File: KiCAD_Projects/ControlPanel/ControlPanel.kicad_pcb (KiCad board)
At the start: 2 copper layers, 0 parts

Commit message: 4.0発注かけた｡テレメトリとコンパネ作る
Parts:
- added D1: LED, LEDs:LED-3MM, F.Cu at (29.2, 3.81)
- added D2: LED, LEDs:LED-3MM, F.Cu at (24.1, 6.35)
- added D3: LED, LEDs:LED-3MM, F.Cu at (29.2, 8.89)
- added D4: LED, LEDs:LED-3MM, F.Cu at (24.1, 11.4)
- added D5: LED, LEDs:LED-3MM, F.Cu at (29.2, 14.0)
- added D6: LED, LEDs:LED-3MM, F.Cu at (24.1, 16.5)
- added D7: LED, LEDs:LED-3MM, F.Cu at (29.2, 19.1)
- added D8: LED, LEDs:LED-3MM, F.Cu at (24.1, 21.6)
- added R1: R, RP_KiCAD_Libs:C1608_WP, B.Cu at (19.1, 3.81)
- added R2: R, RP_KiCAD_Libs:C1608_WP, B.Cu at (19.1, 6.35)
- added R3: R, RP_KiCAD_Libs:C1608_WP, B.Cu at (19.1, 8.89)
- added R4: R, RP_KiCAD_Libs:C1608_WP, B.Cu at (19.1, 11.4)
- added R5: R, RP_KiCAD_Libs:C1608_WP, B.Cu at (19.1, 14.0)
- added R6: R, RP_KiCAD_Libs:C1608_WP, B.Cu at (19.1, 16.5)
- added R7: R, RP_KiCAD_Libs:C1608_WP, B.Cu at (19.1, 19.1)
- added R8: R, RP_KiCAD_Libs:C1608_WP, B.Cu at (19.1, 21.6)
- added SW1: SWITCH_INV, Buttons_Switches_ThroughHole:SW_toggle_3P, F.Cu at (78.7, 2.54)
- added SW2: SWITCH_INV, Buttons_Switches_ThroughHole:SW_toggle_3P, F.Cu at (78.7, 7.62)
- added SW3: SWITCH_INV, Buttons_Switches_ThroughHole:SW_toggle_3P, F.Cu at (78.7, 12.7)
- added SW4: SWITCH_INV, Buttons_Switches_ThroughHole:SW_toggle_3P, F.Cu at (78.7, 17.8)
- added SW5: SWITCH_INV, Buttons_Switches_ThroughHole:SW_toggle_3P, F.Cu at (78.7, 22.9)
- added SW6: SWITCH_INV, Buttons_Switches_ThroughHole:SW_toggle_3P, F.Cu at (78.7, 27.9)
- added SW7: SWITCH_INV, Buttons_Switches_ThroughHole:SW_toggle_3P, F.Cu at (78.7, 33.0)
- added SW8: SWITCH_INV, Buttons_Switches_ThroughHole:SW_toggle_3P, F.Cu at (78.7, 38.1)
- added U1: F103_mini, RP_KiCAD_Libs:F103_mini, F.Cu at (48.3, 25.4)
- added U2: SW_ROTARY_16, Buttons_Switches_ThroughHole:rotary_0F, F.Cu at (22.9, 31.8)
- added U3: SW_ROTARY_16, Buttons_Switches_ThroughHole:rotary_0F, F.Cu at (22.9, 43.2)
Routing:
- net GND: track 0.00 -> 166.6 mm
- net /TOGGLE_H: track 0.00 -> 28.1 mm
- net /TOGGLE_G: track 0.00 -> 25.6 mm
- net /TOGGLE_F: track 0.00 -> 22.3 mm
- net /TOGGLE_E: track 0.00 -> 21.2 mm
- net /TOGGLE_D: track 0.00 -> 20.2 mm
- net /TOGGLE_C: track 0.00 -> 19.1 mm
- net /TOGGLE_B: track 0.00 -> 18.1 mm
- net /TOGGLE_A: track 0.00 -> 18.1 mm
- net /ROTARY_B4: track 0.00 -> 17.1 mm
- net /ROTARY_A4: track 0.00 -> 16.6 mm
- net /ROTARY_B1: track 0.00 -> 16.1 mm
- net /ROTARY_A1: track 0.00 -> 15.5 mm
- net /ROTARY_B8: track 0.00 -> 11.0 mm
- net /ROTARY_A8: track 0.00 -> 10.5 mm
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- added copper zone on B.Cu, net (none)
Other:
- board outline added: 100 x 50 mm

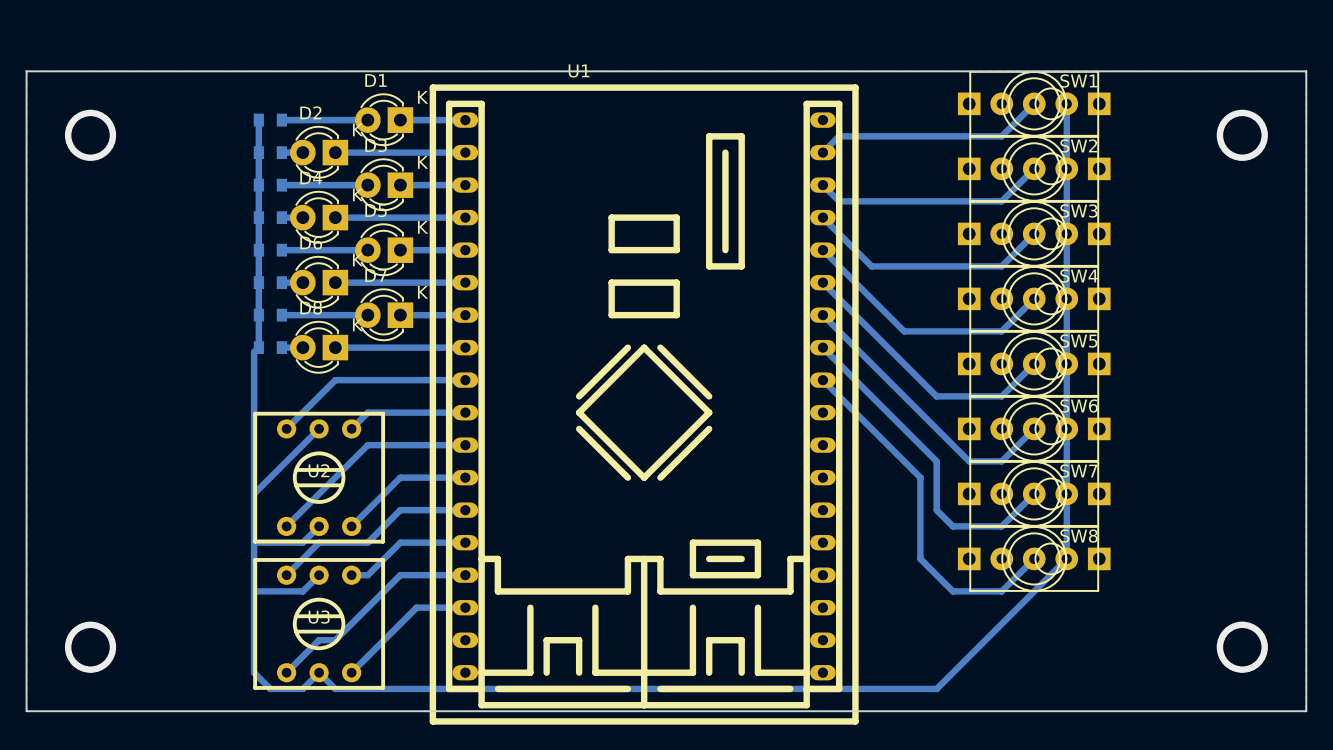
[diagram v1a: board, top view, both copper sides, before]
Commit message: コンパネおわり｡キャンサー作る
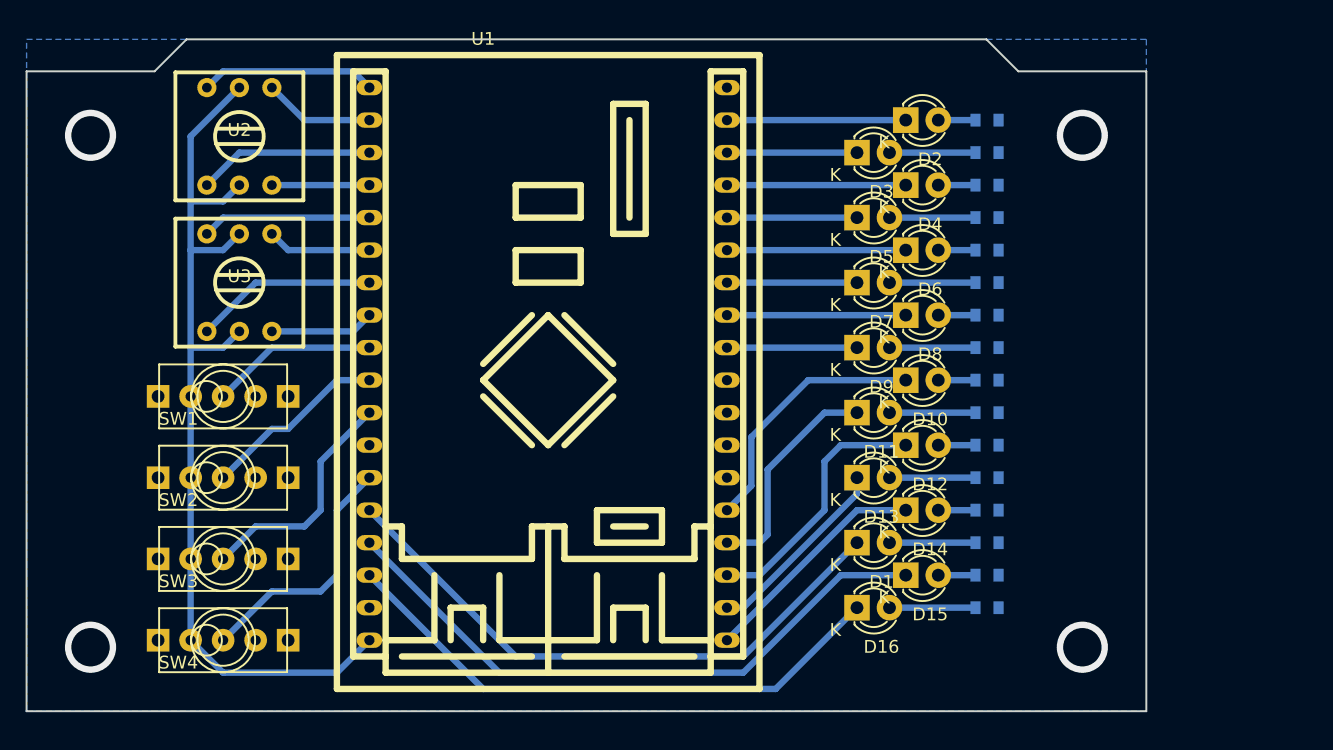
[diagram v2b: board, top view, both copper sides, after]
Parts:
- removed SW5, SW6, SW7, SW8: SWITCH_INV, Buttons_Switches_ThroughHole:SW_toggle_3P
- added D10: LED, LEDs:LED-3MM, F.Cu at (68.7, 24.1)
- added D11: LED, LEDs:LED-3MM, F.Cu at (64.9, 26.7)
- added D12: LED, LEDs:LED-3MM, F.Cu at (68.7, 29.2)
- added D13: LED, LEDs:LED-3MM, F.Cu at (64.9, 31.8)
- added D14: LED, LEDs:LED-3MM, F.Cu at (68.7, 34.3)
- added D15: LED, LEDs:LED-3MM, F.Cu at (68.7, 39.4)
- added D16: LED, LEDs:LED-3MM, F.Cu at (64.9, 41.9)
- added D9: LED, LEDs:LED-3MM, F.Cu at (64.9, 21.6)
- added R10: R, RP_KiCAD_Libs:C1608_WP, B.Cu at (75.0, 24.1)
- added R11: R, RP_KiCAD_Libs:C1608_WP, B.Cu at (75.0, 26.7)
- added R12: R, RP_KiCAD_Libs:C1608_WP, B.Cu at (75.0, 29.2)
- added R13: R, RP_KiCAD_Libs:C1608_WP, B.Cu at (75.0, 31.8)
- added R14: R, RP_KiCAD_Libs:C1608_WP, B.Cu at (75.0, 34.3)
- added R15: R, RP_KiCAD_Libs:C1608_WP, B.Cu at (75.0, 39.4)
- added R16: R, RP_KiCAD_Libs:C1608_WP, B.Cu at (75.0, 41.9)
- added R9: R, RP_KiCAD_Libs:C1608_WP, B.Cu at (75.0, 21.6)
- moved SW4 68.8 mm to (15.4, 44.5), turned to 180 degrees
- moved SW3 68.3 mm to (15.4, 38.1), turned to 180 degrees
- moved SW2 67.8 mm to (15.4, 31.8), turned to 180 degrees
- moved SW1 67.4 mm to (15.4, 25.4), turned to 180 degrees
- moved R1 65.0 mm to (75.0, 36.8), turned to 180 degrees
- moved R2 56.1 mm to (75.0, 3.81), turned to 180 degrees
- moved R3 56.1 mm to (75.0, 6.35), turned to 180 degrees
- moved R4 56.1 mm to (75.0, 8.89), turned to 180 degrees
- moved R5 56.1 mm to (75.0, 11.4), turned to 180 degrees
- moved R6 56.1 mm to (75.0, 14.0), turned to 180 degrees
- moved R7 56.1 mm to (75.0, 16.5), turned to 180 degrees
- moved R8 56.1 mm to (75.0, 19.1), turned to 180 degrees
- moved D1 48.6 mm to (64.9, 36.8), turned to 0 degrees
- moved D2 44.6 mm to (68.7, 3.81), turned to 0 degrees
- moved D4 44.6 mm to (68.7, 8.89), turned to 0 degrees
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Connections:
- U1 pad 1: Net-(D1-Pad1) -> /ROTARY_A1
- U1 pad 10: /ROTARY_A2 -> /TOGGLE_B
- U1 pad 11: /ROTARY_A4 -> /TOGGLE_C
- U1 pad 12: /ROTARY_A8 -> (no net)
- U1 pad 13: /ROTARY_B1 -> /TOGGLE_D
- U1 pad 14: /ROTARY_B2 -> Net-(D1-Pad1)
- U1 pad 15: /ROTARY_B4 -> Net-(D15-Pad1)
- U1 pad 16: /ROTARY_B8 -> Net-(D16-Pad1)
- U1 pad 18: (no net) -> GND
- U1 pad 19: (no net) -> Net-(D14-Pad1)
- U1 pad 2: Net-(D2-Pad1) -> /ROTARY_A2
- U1 pad 20: (no net) -> Net-(D13-Pad1)
- U1 pad 21: (no net) -> Net-(D12-Pad1)
- U1 pad 22: (no net) -> Net-(D11-Pad1)
- U1 pad 23: (no net) -> Net-(D10-Pad1)
- U1 pad 28: /TOGGLE_H -> Net-(D9-Pad1)
- U1 pad 29: /TOGGLE_G -> Net-(D8-Pad1)
- U1 pad 3: Net-(D3-Pad1) -> /ROTARY_A4
- U1 pad 30: /TOGGLE_F -> Net-(D7-Pad1)
- U1 pad 31: /TOGGLE_E -> Net-(D6-Pad1)
- U1 pad 32: /TOGGLE_D -> Net-(D5-Pad1)
- U1 pad 33: /TOGGLE_C -> Net-(D4-Pad1)
- U1 pad 34: /TOGGLE_B -> Net-(D3-Pad1)
- U1 pad 35: /TOGGLE_A -> Net-(D2-Pad1)
- U1 pad 36: (no net) -> GND
- U1 pad 4: Net-(D4-Pad1) -> /ROTARY_A8
- U1 pad 5: Net-(D5-Pad1) -> /ROTARY_B1
- U1 pad 6: Net-(D6-Pad1) -> /ROTARY_B2
- U1 pad 7: Net-(D7-Pad1) -> /ROTARY_B4
- U1 pad 8: Net-(D8-Pad1) -> /ROTARY_B8
- U1 pad 9: /ROTARY_A1 -> /TOGGLE_A
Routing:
- net GND: track 166.6 -> 73.8 mm
- net Net-(D15-Pad1): track 0.00 -> 49.3 mm
- net Net-(D16-Pad1): track 0.00 -> 44.4 mm
- net Net-(D1-Pad1): track 5.08 -> 46.5 mm
- net /TOGGLE_H: track 28.1 -> 0.00 mm
- net /TOGGLE_G: track 25.6 -> 0.00 mm
- net /TOGGLE_F: track 22.3 -> 0.00 mm
- net /TOGGLE_E: track 21.2 -> 0.00 mm
- net Net-(D12-Pad1): track 0.00 -> 20.4 mm
- net Net-(D10-Pad1): track 0.00 -> 20.4 mm
- net Net-(D14-Pad1): track 0.00 -> 18.2 mm
- net Net-(D11-Pad1): track 0.00 -> 17.3 mm
- net Net-(D13-Pad1): track 0.00 -> 15.1 mm
- net Net-(D9-Pad1): track 0.00 -> 10.2 mm
- net Net-(D9-Pad2): track 0.00 -> 6.72 mm
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- added copper zone on B.Cu, net GND
- removed copper zone on B.Cu, net (none)
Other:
- board size 100 x 50 mm -> 87.5 x 52.5 mm
